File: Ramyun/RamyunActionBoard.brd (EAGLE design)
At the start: 133 x 133 mm, 47 parts, among them Q1 BC817-16LT1SMD, U1 PVN012PBF, U10 MAX31856_ADAFRUIT, U11 GPS_ADAFRUIT, U12 BUZZER, U2 PVN012PBF, U3 PVN012PBF, U4 PVN012PBF, U5 PVN012PBF, U6 PVN012PBF, U7 PVN012PBF, U8 PVN012PBF, U9 MAX31856_ADAFRUIT

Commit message: update
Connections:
- new net N$10: R10.2
- new net N$11: R11.2
- new net N$9: R9.2
- net SERVO_1: now also R9.1
- net SERVO_2: now also R10.1
- net SERVO_3: now also R11.1
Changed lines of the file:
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@@
 <signal name="SERVO_2">
 <contactref element="JP1" pad="3"/>
+<contactref element="R10" pad="1"/>
+<wire x1="-253.77" y1="-429.26" x2="-215.78" y2="-278.13" width="0" layer="19" extent="1-1"/>
 </signal>
 <signal name="SERVO_3">
 <contactref element="JP2" pad="3"/>
+<contactref element="R11" pad="1"/>
+<wire x1="-253.77" y1="-433.07" x2="-215.78" y2="-284.48" width="0" layer="19" extent="1-1"/>
 </signal>
 <signal name="SDA">
@@
 <signal name="SERVO_1">
 <contactref element="MS1" pad="21"/>
+<contactref element="R9" pad="1"/>
+<wire x1="-10.16" y1="8.89" x2="-215.78" y2="-271.78" width="0" layer="19" extent="1-1"/>
+</signal>
+<signal name="N$9">
+<contactref element="R9" pad="2"/>
+</signal>
+<signal name="N$10">
+<contactref element="R10" pad="2"/>
+</signal>
+<signal name="N$11">
+<contactref element="R11" pad="2"/>
 </signal>
 </signals>

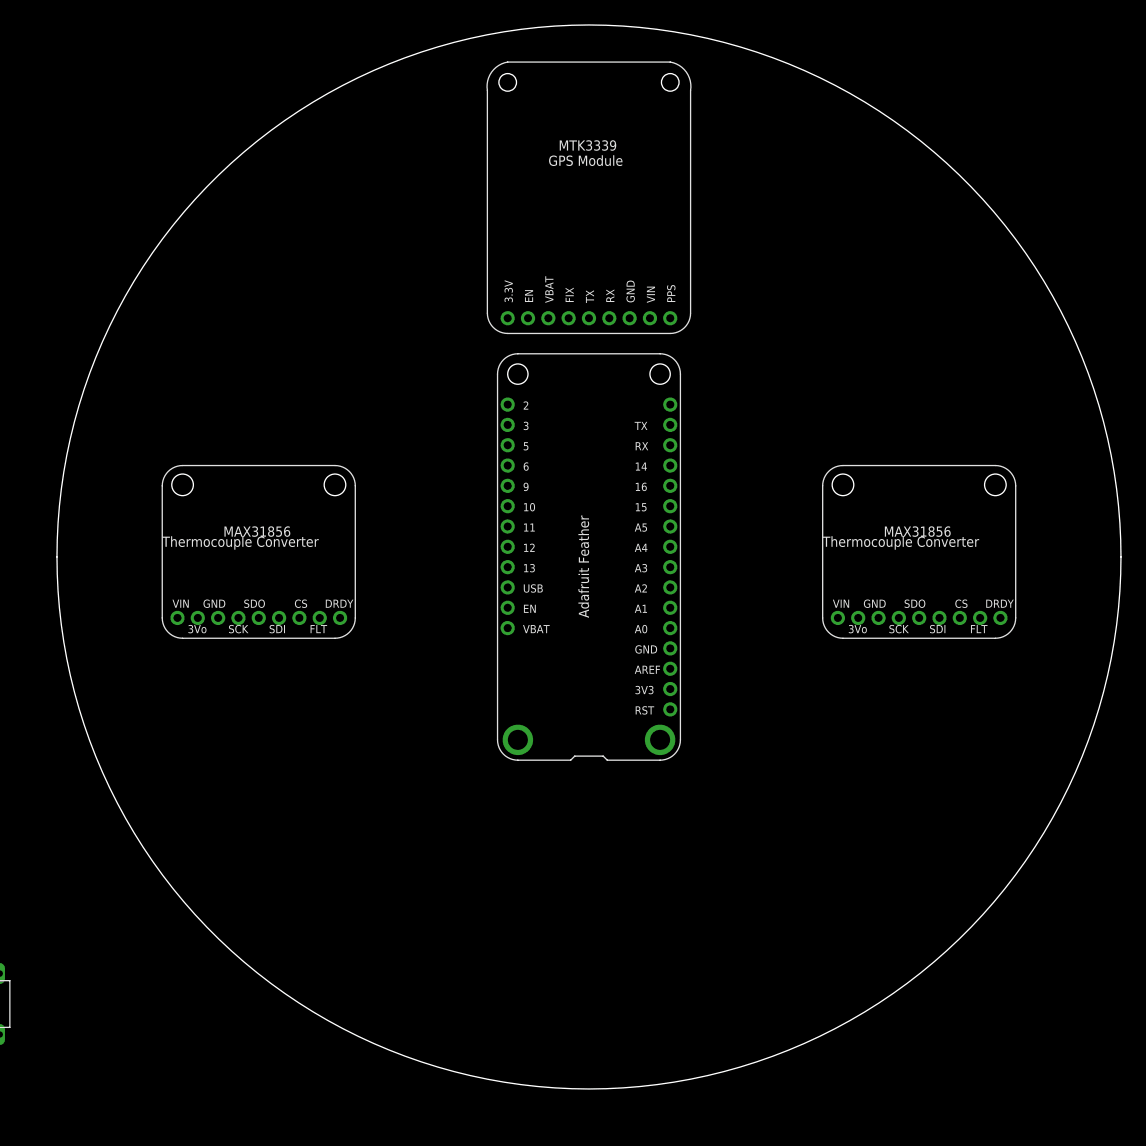
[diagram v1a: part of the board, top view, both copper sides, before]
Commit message: outline
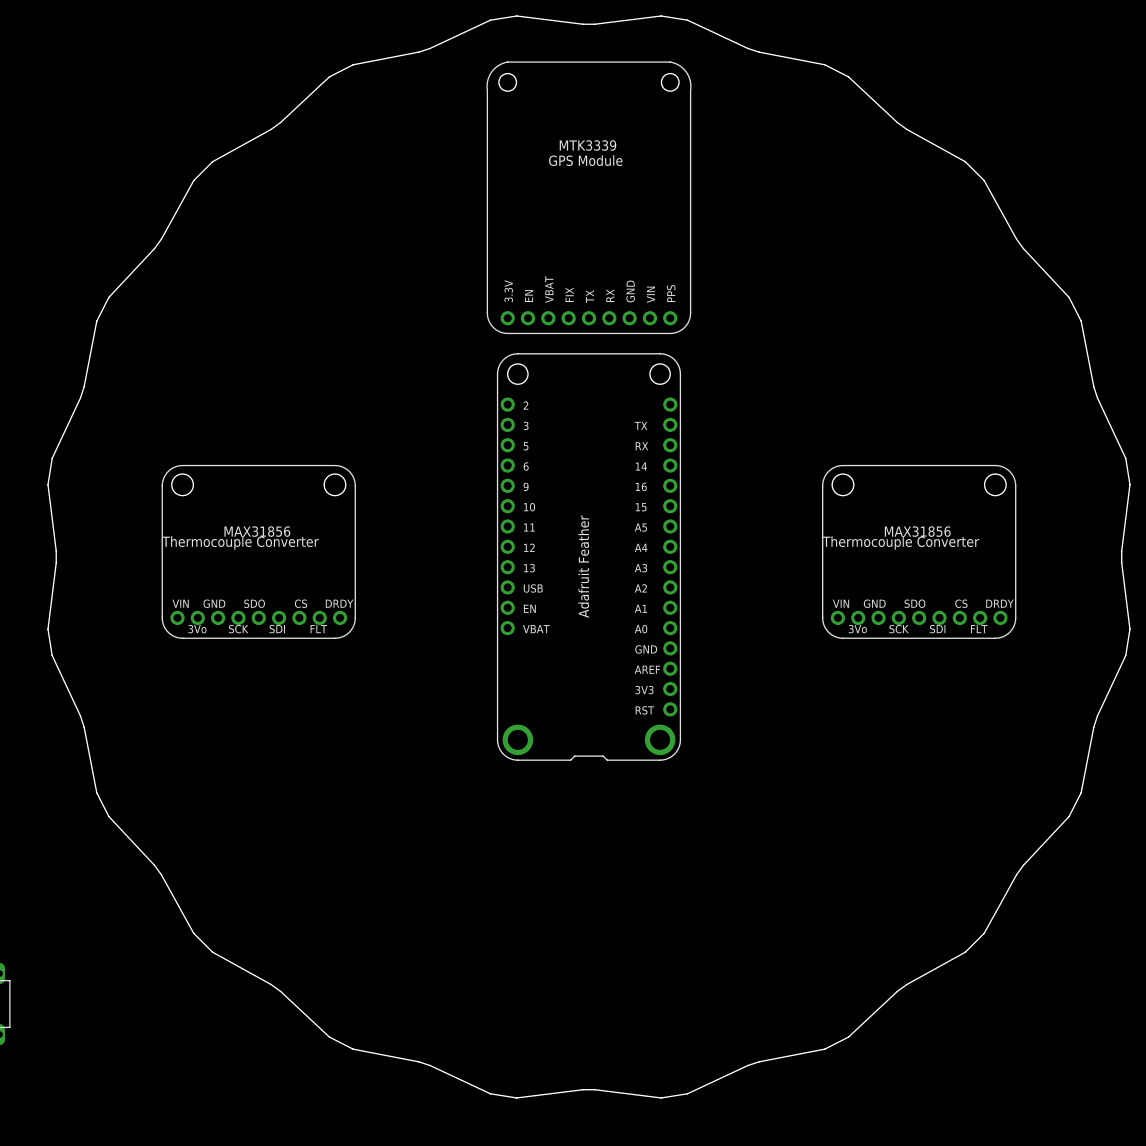
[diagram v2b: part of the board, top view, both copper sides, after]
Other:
- board size 133 x 133 mm -> 135.2 x 135.2 mm
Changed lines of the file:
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@@
 <board>
 <plain>
-<wire x1="66.5" y1="0" x2="-66.5" y2="0" width="0" layer="20" curve="-180"/>
-<wire x1="-66.5" y1="0" x2="66.5" y2="0" width="0" layer="20" curve="-180"/>
+<wire x1="-21.28205" y1="-63.104040625" x2="-19.87408125" y2="-63.56151875" width="0.001" layer="20"/>
+<wire x1="-19.87408125" y1="-63.56151875" x2="-12.311190625" y2="-67.10206875" width="0.001" layer="20"/>
+<wire x1="-12.311190625" y1="-67.10206875" x2="-9.02705" y2="-67.62223125" width="0.001" layer="20"/>
+<wire x1="-9.02705" y1="-67.62223125" x2="-0.740209375" y2="-66.59201875" width="0.001" layer="20"/>
+<wire x1="-0.740209375" y1="-66.59201875" x2="0.740209375" y2="-66.59201875" width="0.001" layer="20"/>
+<wire x1="0.740209375" y1="-66.59201875" x2="9.02705" y2="-67.62223125" width="0.001" layer="20"/>
+<wire x1="9.02705" y1="-67.62223125" x2="12.311190625" y2="-67.10206875" width="0.001" layer="20"/>
+<wire x1="12.311190625" y1="-67.10206875" x2="19.87408125" y2="-63.56151875" width="0.001" layer="20"/>
+<wire x1="19.87408125" y1="-63.56151875" x2="21.28205" y2="-63.104040625" width="0.001" layer="20"/>
+<wire x1="21.28205" y1="-63.104040625" x2="29.48165" y2="-61.52305" width="0.001" layer="20"/>
+<wire x1="29.48165" y1="-61.52305" x2="32.444309375" y2="-60.0135" width="0.001" layer="20"/>
+<wire x1="32.444309375" y1="-60.0135" x2="38.542959375" y2="-54.309159375" width="0.001" layer="20"/>
+<wire x1="38.542959375" y1="-54.309159375" x2="39.74065" y2="-53.438990625" width="0.001" layer="20"/>
+<wire x1="39.74065" y1="-53.438990625" x2="47.050390625" y2="-49.40156875" width="0.001" layer="20"/>
+<wire x1="47.050390625" y1="-49.40156875" x2="49.40156875" y2="-47.050390625" width="0.001" layer="20"/>
+<wire x1="49.40156875" y1="-47.050390625" x2="53.438990625" y2="-39.74065" width="0.001" layer="20"/>
+<wire x1="53.438990625" y1="-39.74065" x2="54.309159375" y2="-38.542959375" width="0.001" layer="20"/>
+<wire x1="54.309159375" y1="-38.542959375" x2="60.0135" y2="-32.444309375" width="0.001" layer="20"/>
+<wire x1="60.0135" y1="-32.444309375" x2="61.52305" y2="-29.48165" width="0.001" layer="20"/>
+<wire x1="61.52305" y1="-29.48165" x2="63.104040625" y2="-21.28205" width="0.001" layer="20"/>
+<wire x1="63.104040625" y1="-21.28205" x2="63.56151875" y2="-19.87408125" width="0.001" layer="20"/>
+<wire x1="63.56151875" y1="-19.87408125" x2="67.10206875" y2="-12.311190625" width="0.001" layer="20"/>
+<wire x1="67.10206875" y1="-12.311190625" x2="67.62223125" y2="-9.02705" width="0.001" layer="20"/>
+<wire x1="67.62223125" y1="-9.02705" x2="66.59201875" y2="-0.740209375" width="0.001" layer="20"/>
+<wire x1="66.59201875" y1="-0.740209375" x2="66.59201875" y2="0.740209375" width="0.001" layer="20"/>
+<wire x1="66.59201875" y1="0.740209375" x2="67.62223125" y2="9.02705" width="0.001" layer="20"/>
+<wire x1="67.62223125" y1="9.02705" x2="67.10206875" y2="12.311190625" width="0.001" layer="20"/>
+<wire x1="67.10206875" y1="12.311190625" x2="63.56151875" y2="19.87408125" width="0.001" layer="20"/>
+<wire x1="63.56151875" y1="19.87408125" x2="63.104040625" y2="21.28205" width="0.001" layer="20"/>
+<wire x1="63.104040625" y1="21.28205" x2="61.52305" y2="29.48165" width="0.001" layer="20"/>
+<wire x1="61.52305" y1="29.48165" x2="60.0135" y2="32.444309375" width="0.001" layer="20"/>
+<wire x1="60.0135" y1="32.444309375" x2="54.309159375" y2="38.542959375" width="0.001" layer="20"/>
+<wire x1="54.309159375" y1="38.542959375" x2="53.438990625" y2="39.74065" width="0.001" layer="20"/>
+<wire x1="53.438990625" y1="39.74065" x2="49.40156875" y2="47.050390625" width="0.001" layer="20"/>
+<wire x1="49.40156875" y1="47.050390625" x2="47.050390625" y2="49.40156875" width="0.001" layer="20"/>
+<wire x1="47.050390625" y1="49.40156875" x2="39.74065" y2="53.438990625" width="0.001" layer="20"/>
+<wire x1="39.74065" y1="53.438990625" x2="38.542959375" y2="54.309159375" width="0.001" layer="20"/>
+<wire x1="38.542959375" y1="54.309159375" x2="32.444309375" y2="60.0135" width="0.001" layer="20"/>
+<wire x1="32.444309375" y1="60.0135" x2="29.48165" y2="61.52305" width="0.001" layer="20"/>
+<wire x1="29.48165" y1="61.52305" x2="21.28205" y2="63.104040625" width="0.001" layer="20"/>
+<wire x1="21.28205" y1="63.104040625" x2="19.87408125" y2="63.56151875" width="0.001" layer="20"/>
+<wire x1="19.87408125" y1="63.56151875" x2="12.311190625" y2="67.10206875" width="0.001" layer="20"/>
+<wire x1="12.311190625" y1="67.10206875" x2="9.02705" y2="67.62223125" width="0.001" layer="20"/>
+<wire x1="9.02705" y1="67.62223125" x2="0.740209375" y2="66.59201875" width="0.001" layer="20"/>
+<wire x1="0.740209375" y1="66.59201875" x2="-0.740209375" y2="66.59201875" width="0.001" layer="20"/>
+<wire x1="-0.740209375" y1="66.59201875" x2="-9.02705" y2="67.62223125" width="0.001" layer="20"/>
+<wire x1="-9.02705" y1="67.62223125" x2="-12.311190625" y2="67.10206875" width="0.001" layer="20"/>
+<wire x1="-12.311190625" y1="67.10206875" x2="-19.87408125" y2="63.56151875" width="0.001" layer="20"/>
+<wire x1="-19.87408125" y1="63.56151875" x2="-21.28205" y2="63.104040625" width="0.001" layer="20"/>
+<wire x1="-21.28205" y1="63.104040625" x2="-29.48165" y2="61.52305" width="0.001" layer="20"/>
+<wire x1="-29.48165" y1="61.52305" x2="-32.444309375" y2="60.0135" width="0.001" layer="20"/>
+<wire x1="-32.444309375" y1="60.0135" x2="-38.542959375" y2="54.309159375" width="0.001" layer="20"/>
+<wire x1="-38.542959375" y1="54.309159375" x2="-39.74065" y2="53.438990625" width="0.001" layer="20"/>
+<wire x1="-39.74065" y1="53.438990625" x2="-47.050390625" y2="49.40156875" width="0.001" layer="20"/>
+<wire x1="-47.050390625" y1="49.40156875" x2="-49.40156875" y2="47.050390625" width="0.001" layer="20"/>
+<wire x1="-49.40156875" y1="47.050390625" x2="-53.438990625" y2="39.74065" width="0.001" layer="20"/>
+<wire x1="-53.438990625" y1="39.74065" x2="-54.309159375" y2="38.542959375" width="0.001" layer="20"/>
+<wire x1="-54.309159375" y1="38.542959375" x2="-60.0135" y2="32.444309375" width="0.001" layer="20"/>
+<wire x1="-60.0135" y1="32.444309375" x2="-61.52305" y2="29.48165" width="0.001" layer="20"/>
+<wire x1="-61.52305" y1="29.48165" x2="-63.104040625" y2="21.28205" width="0.001" layer="20"/>
+<wire x1="-63.104040625" y1="21.28205" x2="-63.56151875" y2="19.87408125" width="0.001" layer="20"/>
+<wire x1="-63.56151875" y1="19.87408125" x2="-67.10206875" y2="12.311190625" width="0.001" layer="20"/>
+<wire x1="-67.10206875" y1="12.311190625" x2="-67.62223125" y2="9.02705" width="0.001" layer="20"/>
+<wire x1="-67.62223125" y1="9.02705" x2="-66.59201875" y2="0.740209375" width="0.001" layer="20"/>
+<wire x1="-66.59201875" y1="0.740209375" x2="-66.59201875" y2="-0.740209375" width="0.001" layer="20"/>
+<wire x1="-66.59201875" y1="-0.740209375" x2="-67.62223125" y2="-9.02705" width="0.001" layer="20"/>
+<wire x1="-67.62223125" y1="-9.02705" x2="-67.10206875" y2="-12.311190625" width="0.001" layer="20"/>
+<wire x1="-67.10206875" y1="-12.311190625" x2="-63.56151875" y2="-19.87408125" width="0.001" layer="20"/>
+<wire x1="-63.56151875" y1="-19.87408125" x2="-63.104040625" y2="-21.28205" width="0.001" layer="20"/>
+<wire x1="-63.104040625" y1="-21.28205" x2="-61.52305" y2="-29.48165" width="0.001" layer="20"/>
+<wire x1="-61.52305" y1="-29.48165" x2="-60.0135" y2="-32.444309375" width="0.001" layer="20"/>
+<wire x1="-60.0135" y1="-32.444309375" x2="-54.309159375" y2="-38.542959375" width="0.001" layer="20"/>
+<wire x1="-54.309159375" y1="-38.542959375" x2="-53.438990625" y2="-39.74065" width="0.001" layer="20"/>
+<wire x1="-53.438990625" y1="-39.74065" x2="-49.40156875" y2="-47.050390625" width="0.001" layer="20"/>
+<wire x1="-49.40156875" y1="-47.050390625" x2="-47.050390625" y2="-49.40156875" width="0.001" layer="20"/>
+<wire x1="-47.050390625" y1="-49.40156875" x2="-39.74065" y2="-53.438990625" width="0.001" layer="20"/>
+<wire x1="-39.74065" y1="-53.438990625" x2="-38.542959375" y2="-54.309159375" width="0.001" layer="20"/>
+<wire x1="-38.542959375" y1="-54.309159375" x2="-32.444309375" y2="-60.0135" width="0.001" layer="20"/>
+<wire x1="-32.444309375" y1="-60.0135" x2="-29.48165" y2="-61.52305" width="0.001" layer="20"/>
+<wire x1="-29.48165" y1="-61.52305" x2="-21.28205" y2="-63.104040625" width="0.001" layer="20"/>
 </plain>
 <attributes>
